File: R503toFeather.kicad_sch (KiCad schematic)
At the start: 4 parts, among them J1 MX1.0 6P

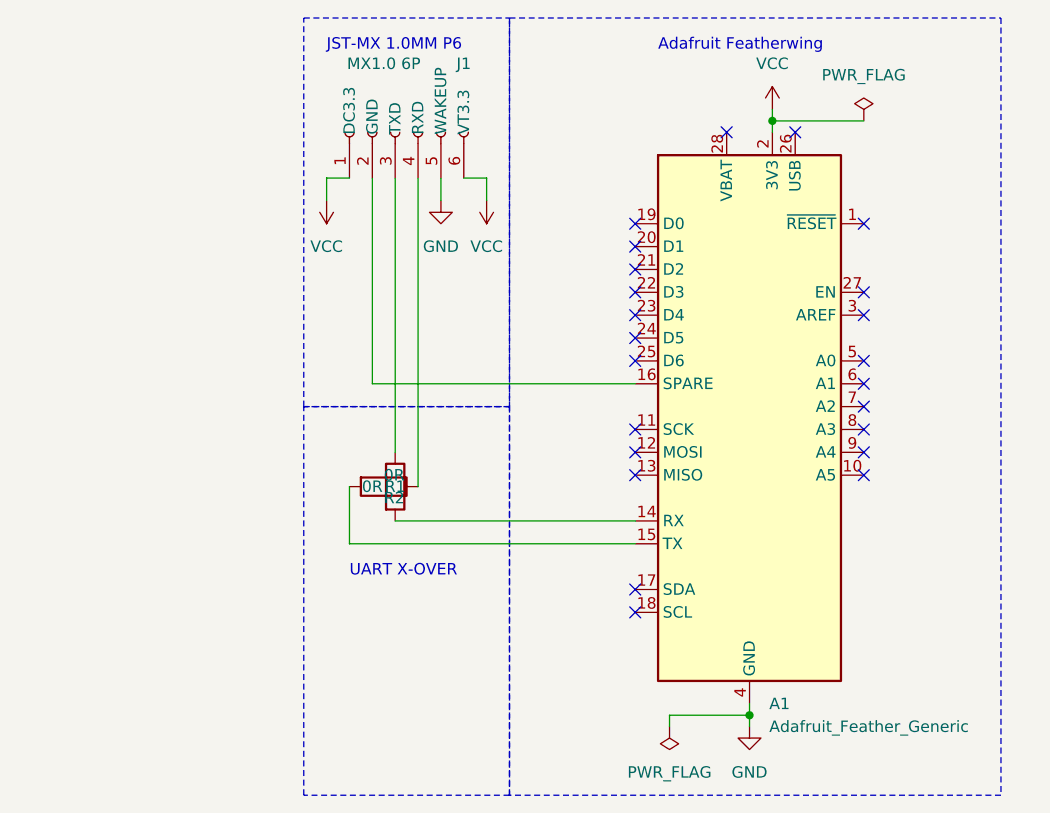
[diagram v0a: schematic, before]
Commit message: RP2350 HSTX Production Version
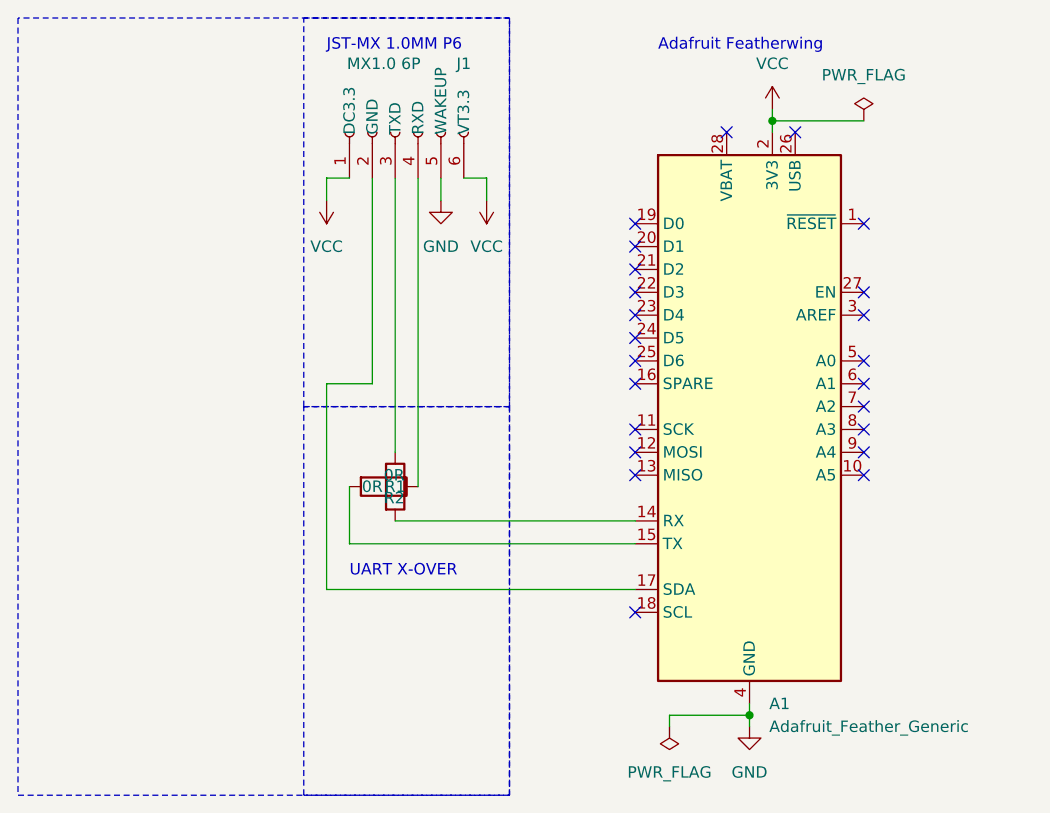
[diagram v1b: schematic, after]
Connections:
- net at A1.16 (SPARE): no longer J1.2 (GND)
- net at A1.17 (SDA): now also J1.2 (GND)
